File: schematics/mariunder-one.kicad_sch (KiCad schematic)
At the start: 44 parts, among them J1 Conn_01x07_I2S, J2 USB_A, J3 Conn_01x02, J4 Conn_02x04_C1101, Q1 2N3904, SW1 SW_Push_Dual_UP, SW10 SW_Push_Dual_BTN_A, SW11 SW_SPDT, SW2 SW_Push_Dual_DOWN, SW3 SW_Push_Dual_LEFT, SW4 SW_Push_Dual_RIGHT, SW5 SW_Push_Dual_MENU, SW6 SW_Push_VOLUME, SW7 SW_Push_Dual_SELECT, SW8 SW_Push_Dual_START, SW9 SW_Push_Dual_BTN_B, U1 ESP32-S3-DevKitC, U2 TFT_320x240

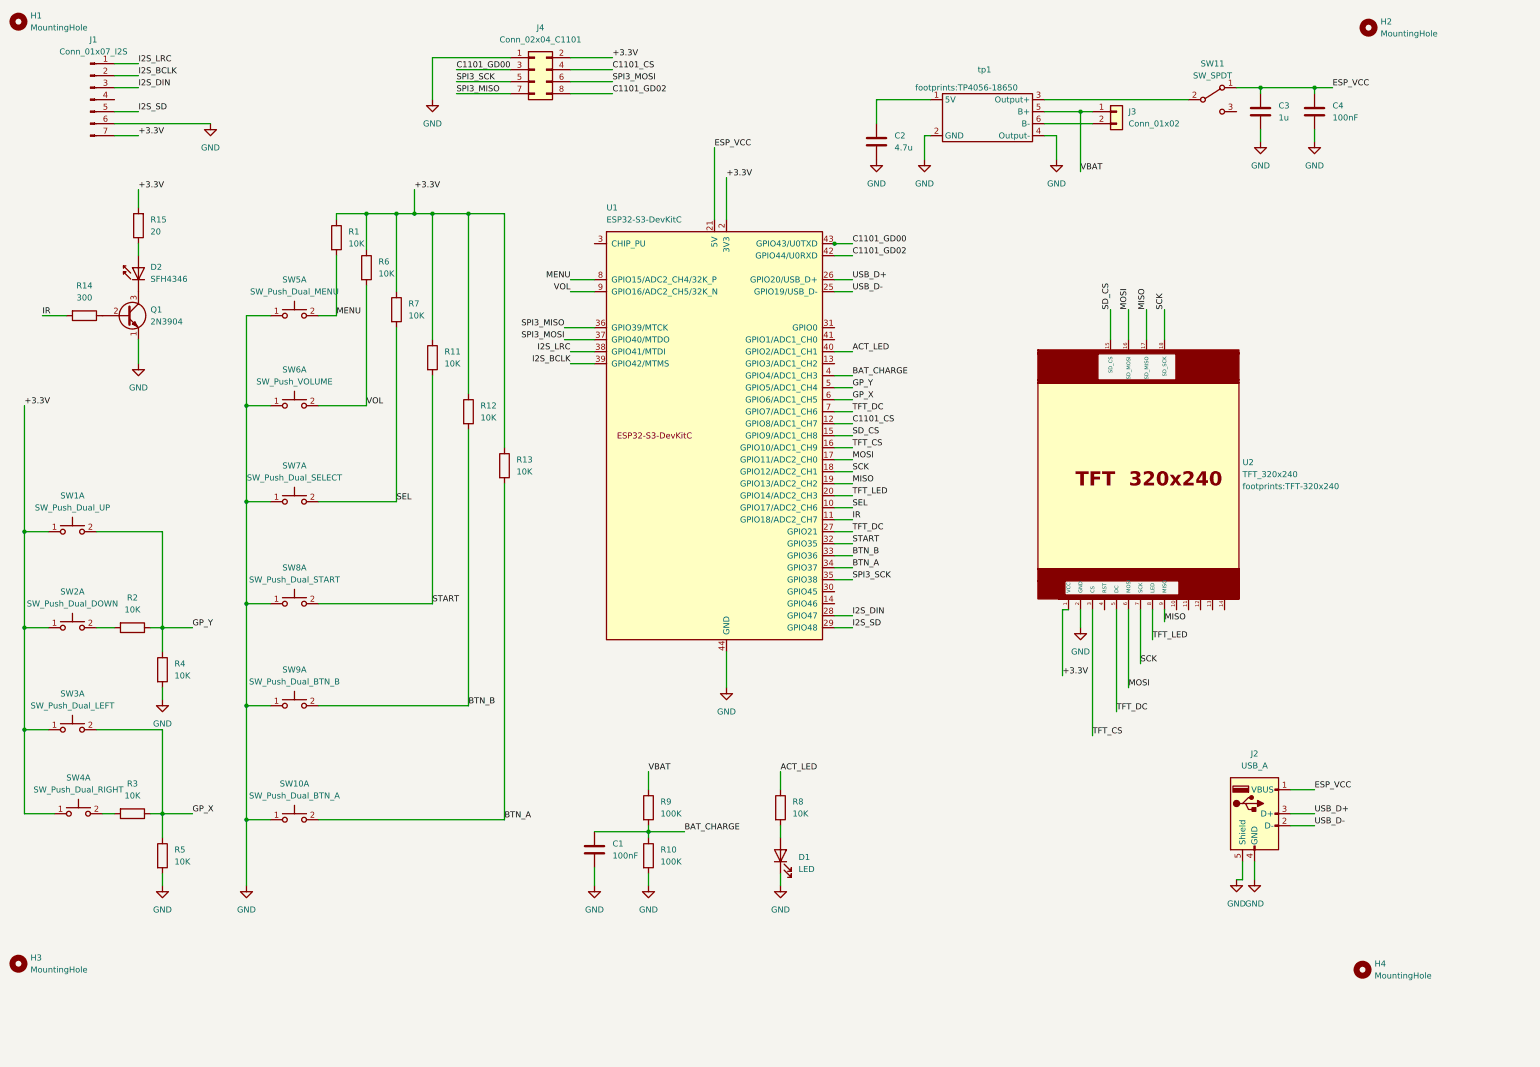
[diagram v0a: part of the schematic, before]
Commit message: updated project structure
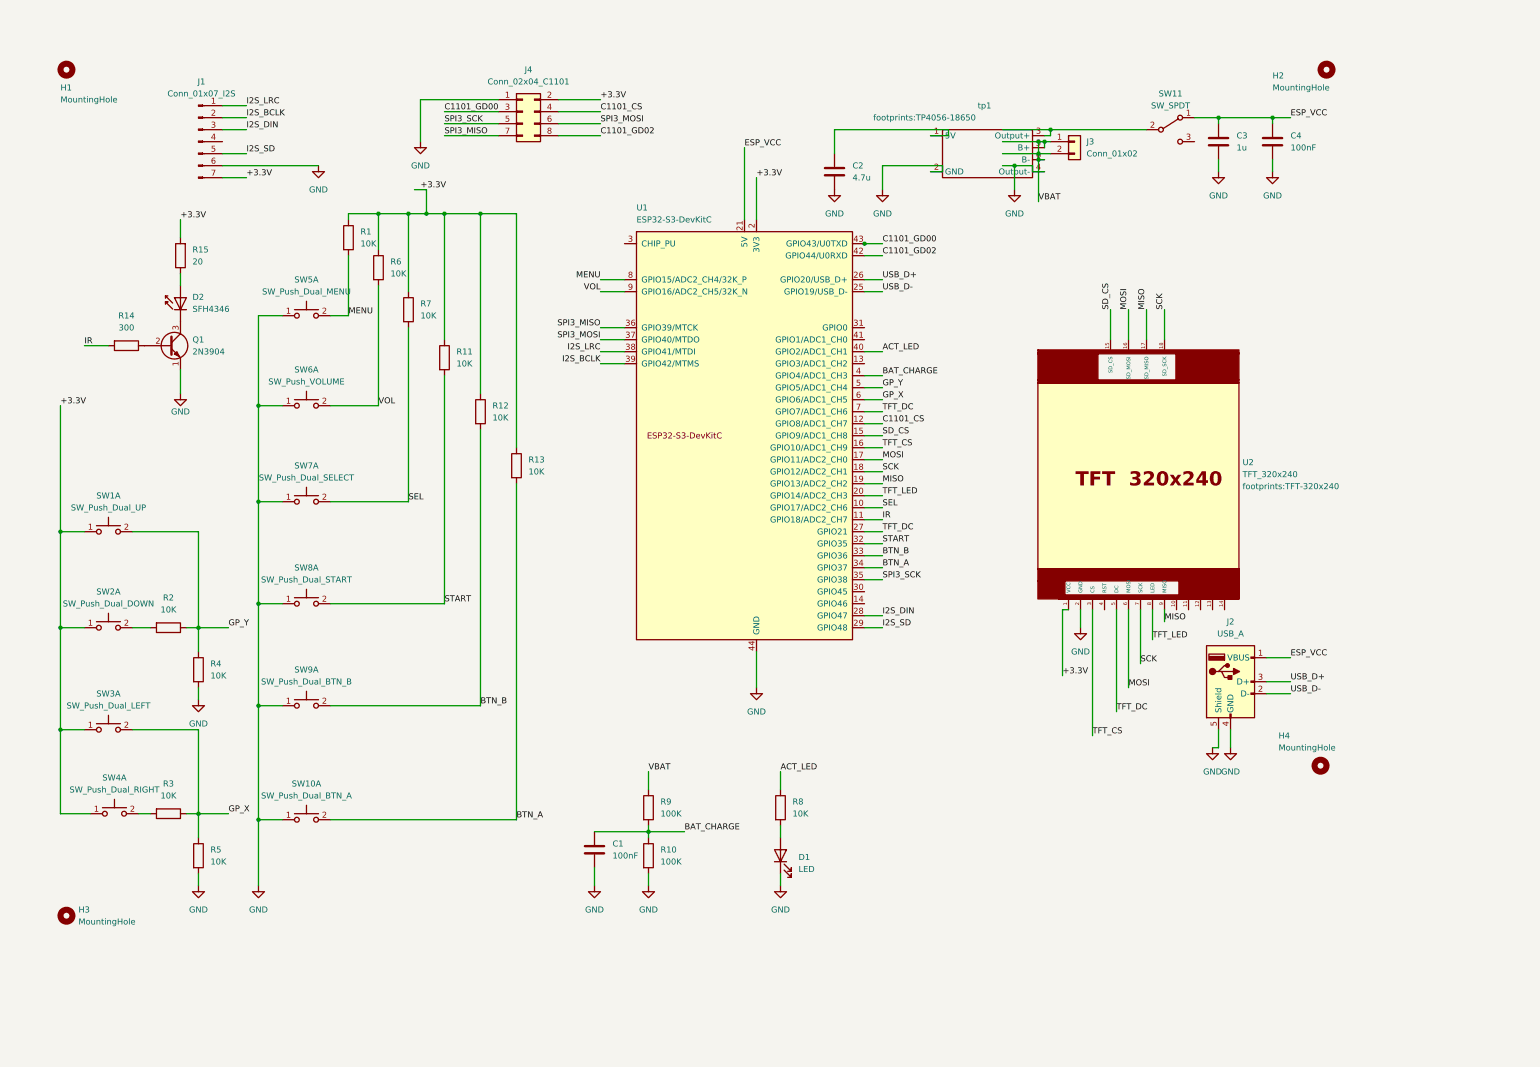
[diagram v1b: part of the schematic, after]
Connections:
- net VBAT: now also J3.2 (Pin_2), tp1.6 (B-)
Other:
- moved on the sheet: C2, C3, C4, D2, H1, H2, H3, H4, J1, J2, J3, J4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
